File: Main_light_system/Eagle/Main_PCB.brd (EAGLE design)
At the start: 104 x 50 mm, 20 parts, among them J1 Vin, U1 TPS54308DDCT, U2 TPS54308DDCT

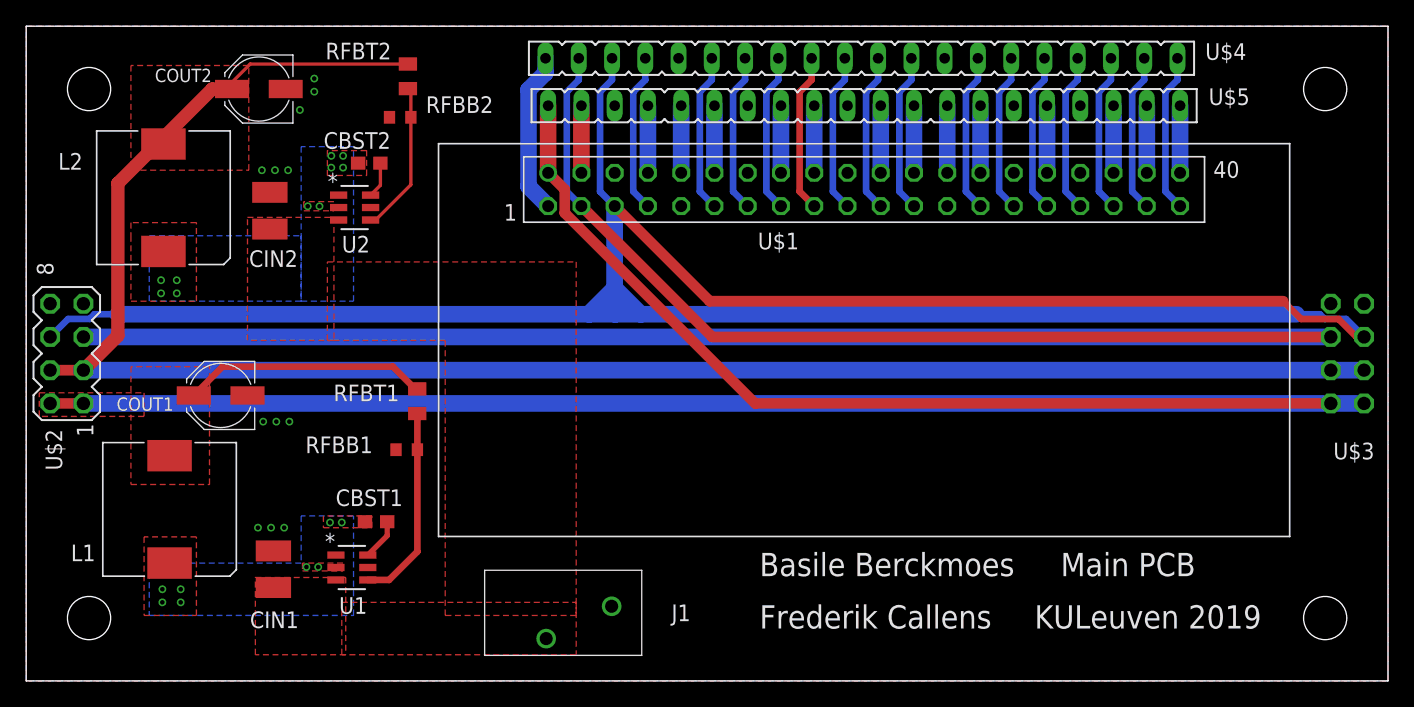
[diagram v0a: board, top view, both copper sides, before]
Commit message: pcb update
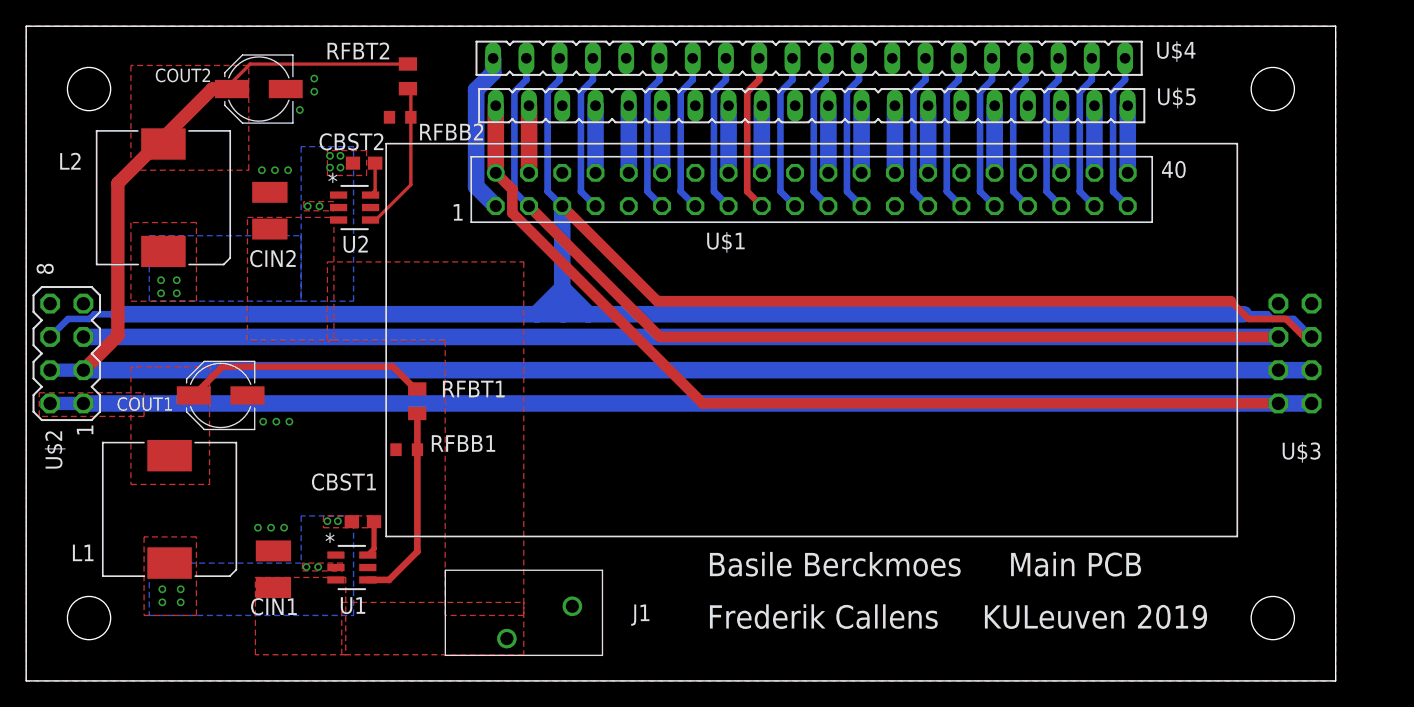
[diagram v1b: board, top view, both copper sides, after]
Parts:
- moved U$1 4.00 mm to (60.0, 37.5)
- moved U$3 4.00 mm to (96.9, 25.0)
- moved U$4 4.00 mm to (59.8, 47.5)
- moved U$5 4.00 mm to (60.0, 43.9)
- moved J1 3.00 mm to (44.0, 4.45)
- moved CBST1 1.00 mm to (25.7, 12.2)
- moved CBST2 0.40 mm to (25.8, 39.5)
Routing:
- net 5V: track 192.3 -> 188.3 mm
- net SDA: track 168.8 -> 164.8 mm
- net SCL: track 189.2 -> 185.2 mm
- net 3.3V: track 141.9 -> 137.9 mm
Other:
- board size 104 x 50 mm -> 100 x 50 mm

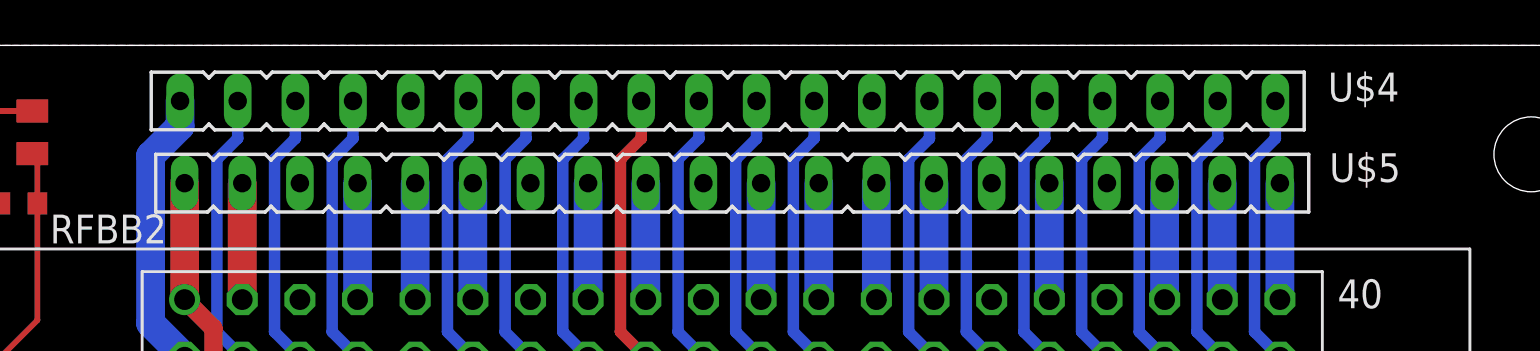
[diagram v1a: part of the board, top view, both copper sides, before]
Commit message: gerbers r2order
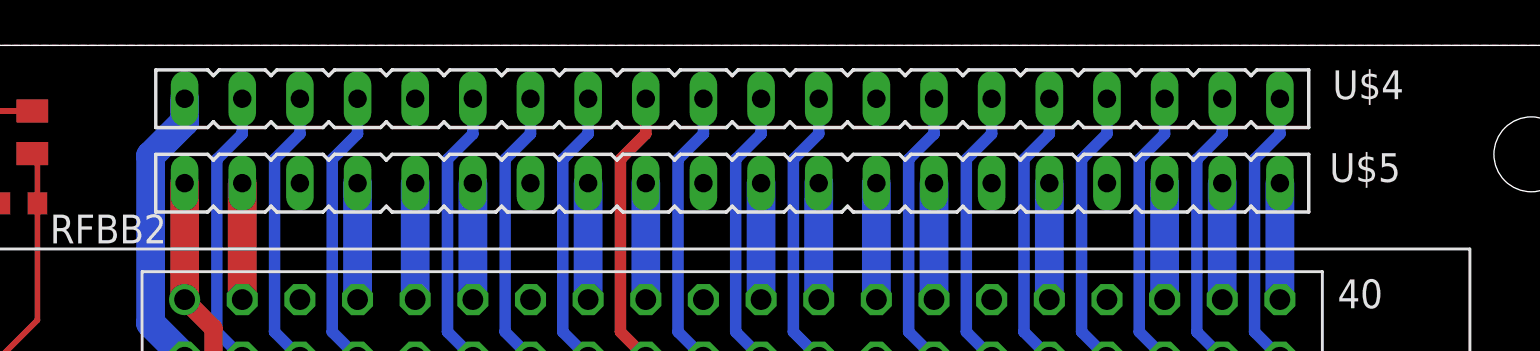
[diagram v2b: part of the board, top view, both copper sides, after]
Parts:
- moved U$4 0.22 mm to (60.0, 47.6)
